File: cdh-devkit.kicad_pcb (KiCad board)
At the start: 4 copper layers, 45 x 80 mm, 37 parts, among them J1 SWD, J2 Conn_01x15_Male, J3 Conn_01x09_Male, J4 USB_B_Micro, U1 AMS1117-3.3, U2 STM32L433RCT6, U3 MX25V8035FM2I, U4 DS1339U-33+T&R, Y1 16MHz, Y2 32.768K

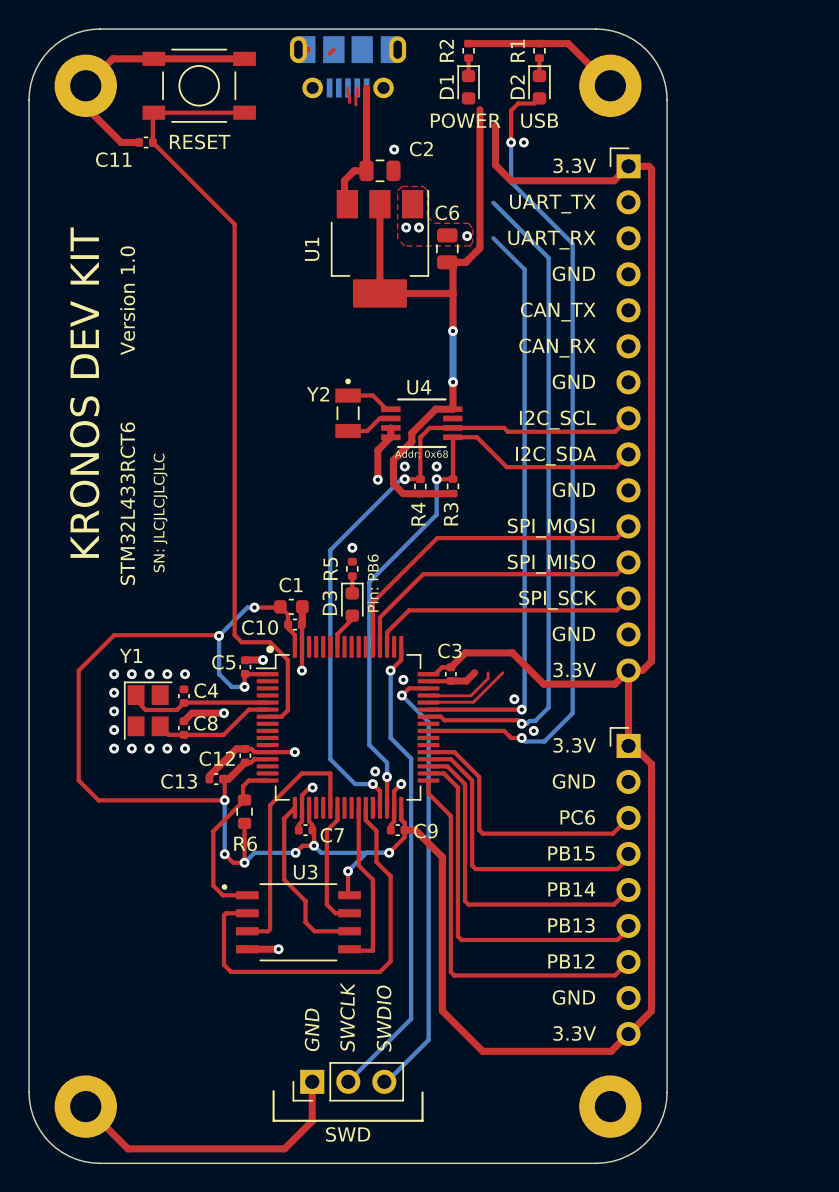
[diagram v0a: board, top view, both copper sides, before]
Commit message: finished second revision
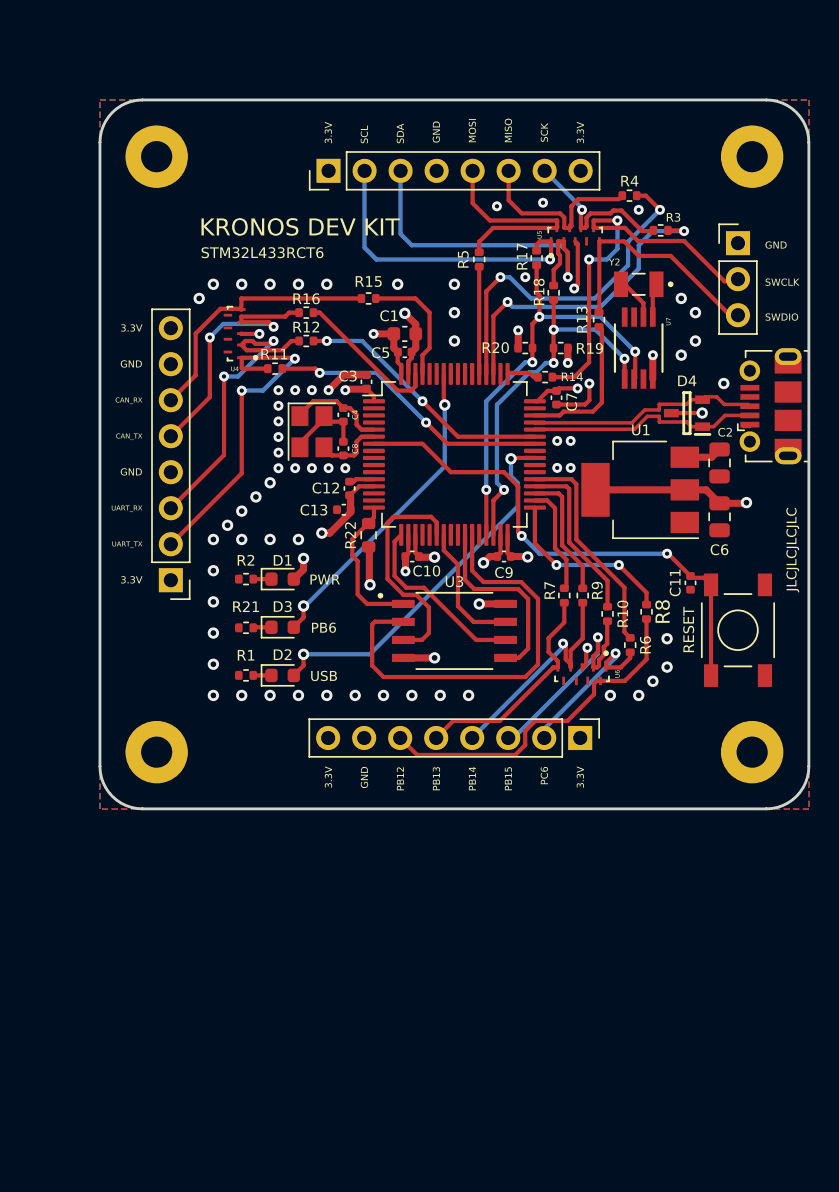
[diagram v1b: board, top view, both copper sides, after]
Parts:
- added D4: PESD2USB3UV-TR, TVS:SOT95P230X110-3N, F.Cu at (61.4, 42.1)
- added J5: SWD, Connector_PinHeader_2.54mm:PinHeader_1x03_P2.54mm_Vertical, F.Cu at (65.0, 30.1)
- added R10: 1K, Resistor_SMD:R_0402_1005Metric, F.Cu at (55.8, 56.2)
- added R11: 1K, Resistor_SMD:R_0402_1005Metric, F.Cu at (32.4, 39.0)
- added R12: 1K, Resistor_SMD:R_0402_1005Metric, F.Cu at (34.5, 37.0)
- added R13: 1K, Resistor_SMD:R_0402_1005Metric, F.Cu at (55.2, 35.5)
- added R14: 1K, Resistor_SMD:R_0402_1005Metric, F.Cu at (51.4, 39.5)
- added R15: 1K, Resistor_SMD:R_0402_1005Metric, F.Cu at (39.0, 34.0)
- added R16: 1K, Resistor_SMD:R_0402_1005Metric, F.Cu at (34.5, 35.0)
- added R17: 1K, Resistor_SMD:R_0402_1005Metric, F.Cu at (50.8, 31.1)
- added R18: 1K, Resistor_SMD:R_0402_1005Metric, F.Cu at (52.0, 33.6)
- added R19: 10k, Resistor_SMD:R_0402_1005Metric, F.Cu at (52.5, 37.5)
- added R20: 10k, Resistor_SMD:R_0402_1005Metric, F.Cu at (50.0, 37.5)
- added R21: 1k5, Resistor_SMD:R_0402_1005Metric, F.Cu at (30.3, 57.2)
- added R22: 10K, Resistor_SMD:R_0603_1608Metric, F.Cu at (39.0, 50.7)
- added R7: 1K, Resistor_SMD:R_0402_1005Metric, F.Cu at (52.8, 55.0)
- added R8: 1K, Resistor_SMD:R_0402_1005Metric, F.Cu at (58.5, 56.1)
- added R9: 1K, Resistor_SMD:R_0402_1005Metric, F.Cu at (54.0, 55.0)
- added U5: DT1240A-08LP3810-7, TVS:TVS_824014883, F.Cu at (53.5, 29.5)
- added U6: DT1240A-08LP3810-7, TVS:TVS_824014883, F.Cu at (54.0, 60.5)
- added U7: DS1339U-33+T&R, MSOP:21-0036K, F.Cu at (58.0, 37.5)
- J1: value SWD -> Conn_01x08_Male; footprint Connector_PinHeader_2.54mm:PinHeader_1x03_P2.54mm_Vertical -> Connector_PinHeader_2.54mm:PinHeader_1x08_P2.54mm_Vertical
- J2: value Conn_01x15_Male -> Conn_01x08_Male; footprint Connector_PinHeader_2.54mm:PinHeader_1x15_P2.54mm_Horizontal -> Connector_PinHeader_2.54mm:PinHeader_1x08_P2.54mm_Vertical
- J3: value Conn_01x09_Male -> Conn_01x08_Male; footprint Connector_PinHeader_2.54mm:PinHeader_1x09_P2.54mm_Horizontal -> Connector_PinHeader_2.54mm:PinHeader_1x08_P2.54mm_Vertical
- J4: moved to F.Cu
- R3, R4, R5: value 1k5 -> 1K
- R6: value 10K -> 1K; footprint Resistor_SMD:R_0603_1608Metric -> Resistor_SMD:R_0402_1005Metric
- U4: value DS1339U-33+T&R -> DT1240A-08LP3810-7; footprint MSOP:21-0036K -> TVS:TVS_824014883
- moved H2 67.7 mm to (66.0, 24.0)
- moved H3 56.9 mm to (24.0, 66.0)
- moved S1 54.0 mm to (65.0, 57.4), turned to 90 degrees
- moved H4 53.2 mm to (66.0, 66.0)
- moved C11 49.4 mm to (61.6, 54.1), turned to -90 degrees
- moved R1 48.7 mm to (30.3, 60.6), turned to 180 degrees
- moved D2 45.3 mm to (32.9, 60.6), turned to 0 degrees
- moved R2 40.4 mm to (30.3, 53.8), turned to 180 degrees
- moved J4 38.2 mm to (67.3, 41.6), turned to 90 degrees
- moved D1 37.1 mm to (32.9, 53.8), turned to 0 degrees
- moved J1 36.8 mm to (25.0, 53.9), turned to 180 degrees
- moved C7 35.3 mm to (52.2, 41.0), turned to -90 degrees
- moved C2 31.6 mm to (63.7, 45.6), turned to -90 degrees
- moved R6 29.6 mm to (57.4, 58.5), turned to -90 degrees
- moved C6 26.9 mm to (63.7, 49.4), turned to -90 degrees
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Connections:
- J1 pad 1: GND -> +3.3V
- J1 pad 2: SWCLK -> UART_TX
- J1 pad 3: SWDIO -> UART_RX
- J2 pad 2: UART_TX -> I2C_SCL
- J2 pad 3: UART_RX -> I2C_SDA
- J2 pad 5: CAN_TX -> SPI_MOSI
- J2 pad 6: CAN_RX -> SPI_MISO
- J2 pad 7: GND -> SPI_SCK
- J2 pad 8: I2C_SCL -> +3.3V
- J3 pad 2: GND -> GPIO_1
- J3 pad 3: GPIO_1 -> GPIO_2
- J3 pad 4: GPIO_2 -> GPIO_3
- J3 pad 5: GPIO_3 -> GPIO_4
- J3 pad 6: GPIO_4 -> GPIO_5
- J3 pad 7: GPIO_5 -> GND
- J3 pad 8: GND -> +3.3V
- R3 pad 1: I2C_SDA -> SPI_SCK
- R3 pad 2: +3.3V -> SPI_SCK
- R4 pad 1: I2C_SCL -> SPI_MISO
- R4 pad 2: +3.3V -> SPI_MISO
- R5 pad 1: /GPIO_LED_K -> SPI_MOSI
- R5 pad 2: GND -> SPI_MOSI
- R6 pad 1: +3.3V -> GPIO_1
- R6 pad 2: QSPI_NCS -> GPIO_1
- U4 pad 1: Net-(U4-Pad1) -> UART_TX
- U4 pad 2: Net-(U4-Pad2) -> UART_RX
- U4 pad 4: GND -> CAN_TX
- U4 pad 5: I2C_SDA -> CAN_RX
- U4 pad 6: I2C_SCL -> unconnected-(U4-Pad6)
- U4 pad 8: +3.3V -> unconnected-(U4-Pad8)
- Y2 pad 1: Net-(U4-Pad1) -> Net-(U7-Pad1)
- Y2 pad 2: Net-(U4-Pad2) -> Net-(U7-Pad2)
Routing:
- net +3.3V: track 252.7 -> 43.4 mm, vias 12 -> 13
- net GND: track 84.1 -> 35.3 mm, vias 33 -> 72
- net /USB_NOE: track 58.0 -> 26.3 mm
- net CAN_TX: track 0.00 -> 30.5 mm, vias 0 -> 2
- net CAN_RX: track 0.00 -> 27.4 mm
- net /GPIO_LED: track 2.63 -> 22.3 mm, vias 0 -> 2
- net Net-(C11-Pad1): track 55.3 -> 36.2 mm, vias 0 -> 2
- net SPI_MISO: track 21.2 -> 37.8 mm, vias 0 -> 2
- net SPI_SCK: track 19.0 -> 34.2 mm, vias 0 -> 3
- net D+: track 6.20 -> 16.4 mm
- net GPIO_5: track 27.2 -> 37.2 mm, vias 0 -> 2
- net D-: track 7.38 -> 16.4 mm
- net I2C_SDA: track 43.4 -> 51.6 mm, vias 2 -> 5
- net GPIO_1: track 19.1 -> 27.2 mm, vias 0 -> 1
- net GPIO_2: track 21.4 -> 28.0 mm, vias 0 -> 1
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- added copper zone on In2.Cu, net +3.3V
- added copper zone on B.Cu, net GND
- removed copper zone on In2.Cu, net GND
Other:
- board size 45 x 80 mm -> 50 x 50 mm
- board text added: "JLCJLCJLCJLC"
- board text added: "MISO"
- board text added: "MOSI"
- board text added: "PB6"
- board text added: "PWR"
- board text added: "SCK"
- board text added: "SCL"
- board text added: "SDA"
- board text added: "U1"
- board text removed: "Addr: 0x68"
- board text removed: "I2C_SCL"
- board text removed: "I2C_SDA"
- board text removed: "POWER"
- board text removed: "Pin: PB6"
- board text removed: "SN: JLCJLCJLCJLC"
- board text removed: "SPI_MISO"
- board text removed: "SPI_MOSI"
- board text removed: "SPI_SCK"
- board text removed: "SWD"
- board text removed: "Version 1.0"
